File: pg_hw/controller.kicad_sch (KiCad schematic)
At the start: 29 parts, among them J1 USB_B_Micro, Q1 SS8050, Q2 SS8050, SW1 SW_MEC_5E, SW2 SW_MEC_5E, U1 BW16, U12 MIC29302AWU, U2 MIC29302AWU, U3 CH340C, U7 PCF8574A

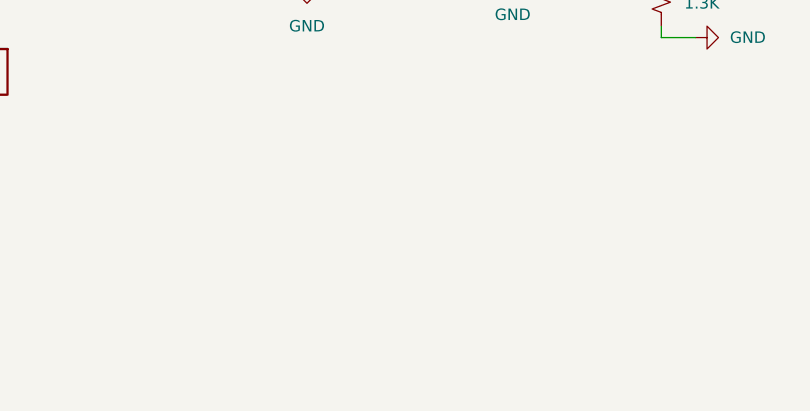
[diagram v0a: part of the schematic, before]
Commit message: ahzeq
ahzeq
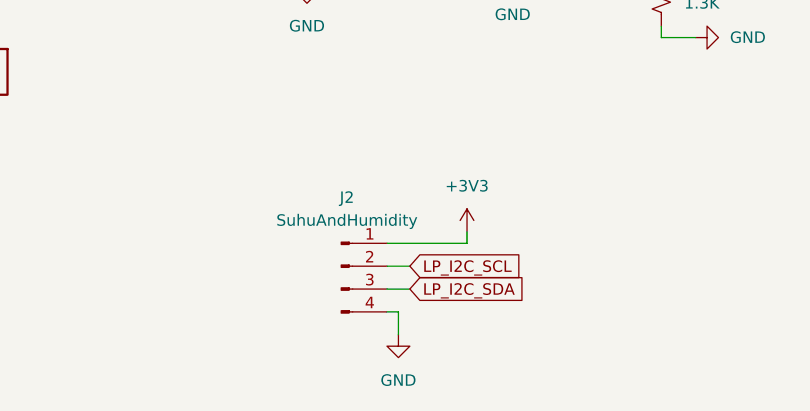
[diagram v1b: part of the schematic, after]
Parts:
- added J2: SuhuAndHumidity, symbol Connector:Conn_01x04_Pin
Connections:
- net +3V3: now also J2.1 (Pin_1)
- net CTP_SCL: now also J2.2 (Pin_2)
- net CTP_SDA: now also J2.3 (Pin_3)
- net GND: now also J2.4 (Pin_4)
